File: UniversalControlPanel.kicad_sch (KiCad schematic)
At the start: 46 parts, among them J1 USB_B_Micro, J10 Conn_01x02, J11 Conn_01x02, J2 Conn_ARM_JTAG_SWD_10, J3 Conn_01x40, J4 Conn_02x03_Odd_Even, J5 Conn_01x02, J6 1Wire, J7 Conn_01x06, J8 Conn_01x07, J9 Conn_01x02, SW1 SW_Push, U1 TSR_1-2450, U2 MAX14783ExS, U3 USBLC6-2SC6, U4 AMS1117-3.3, U5 SN65HVD230, U6 ESP32-S2-WROOM-I

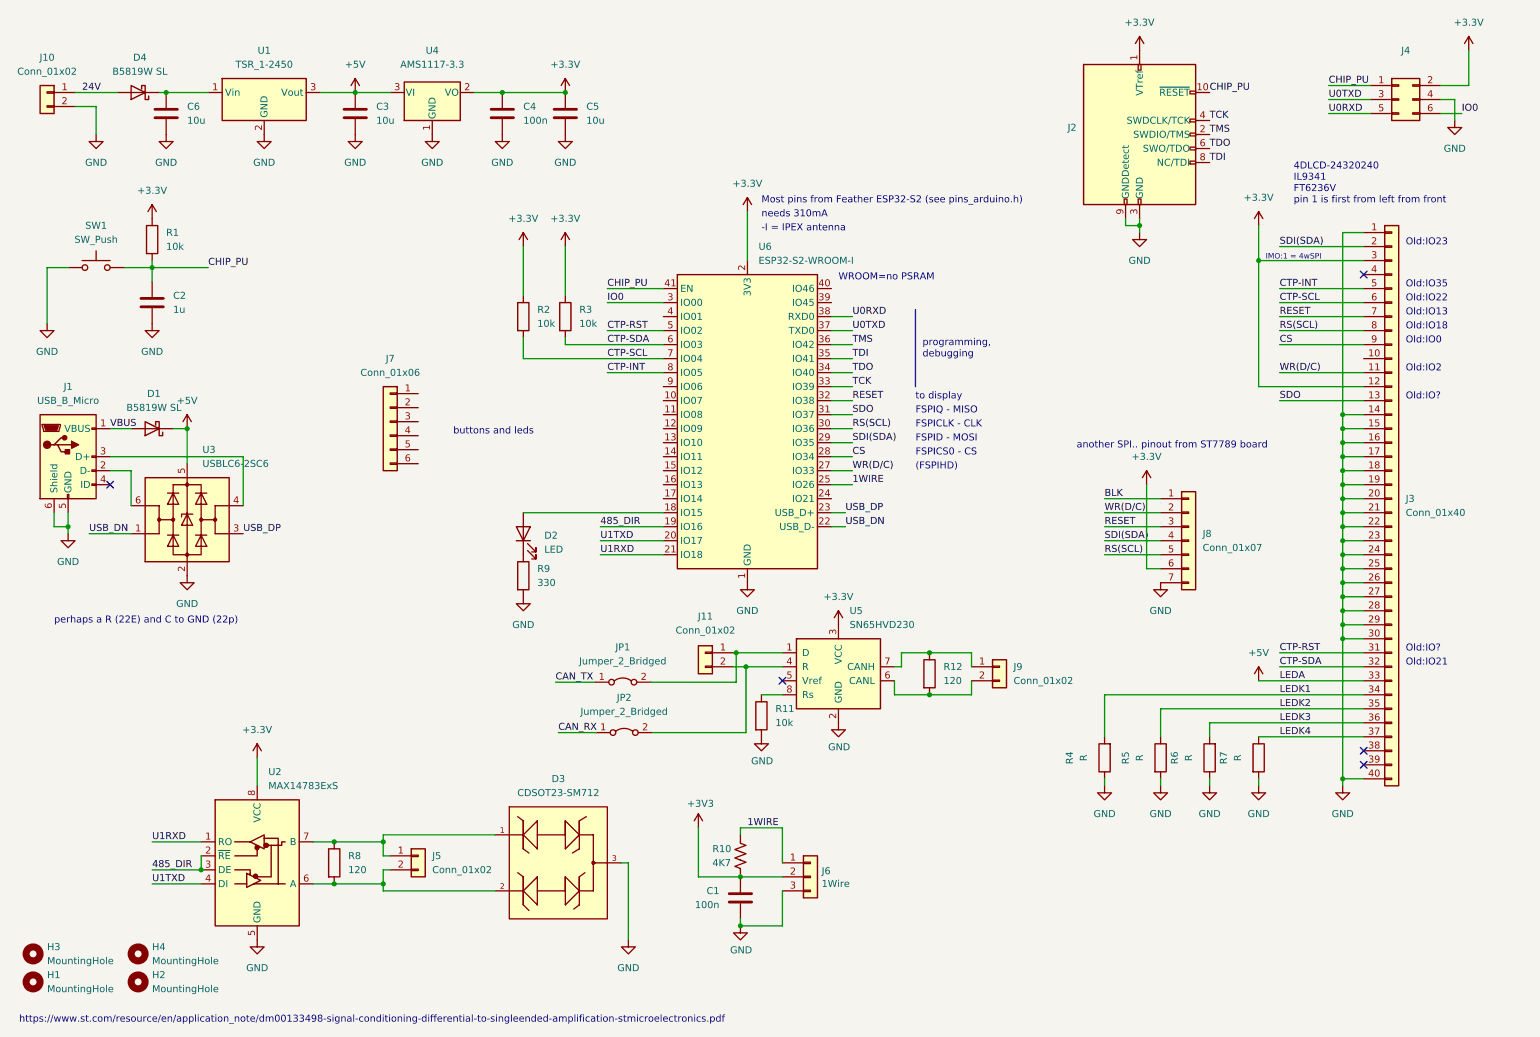
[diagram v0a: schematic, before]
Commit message: restart work
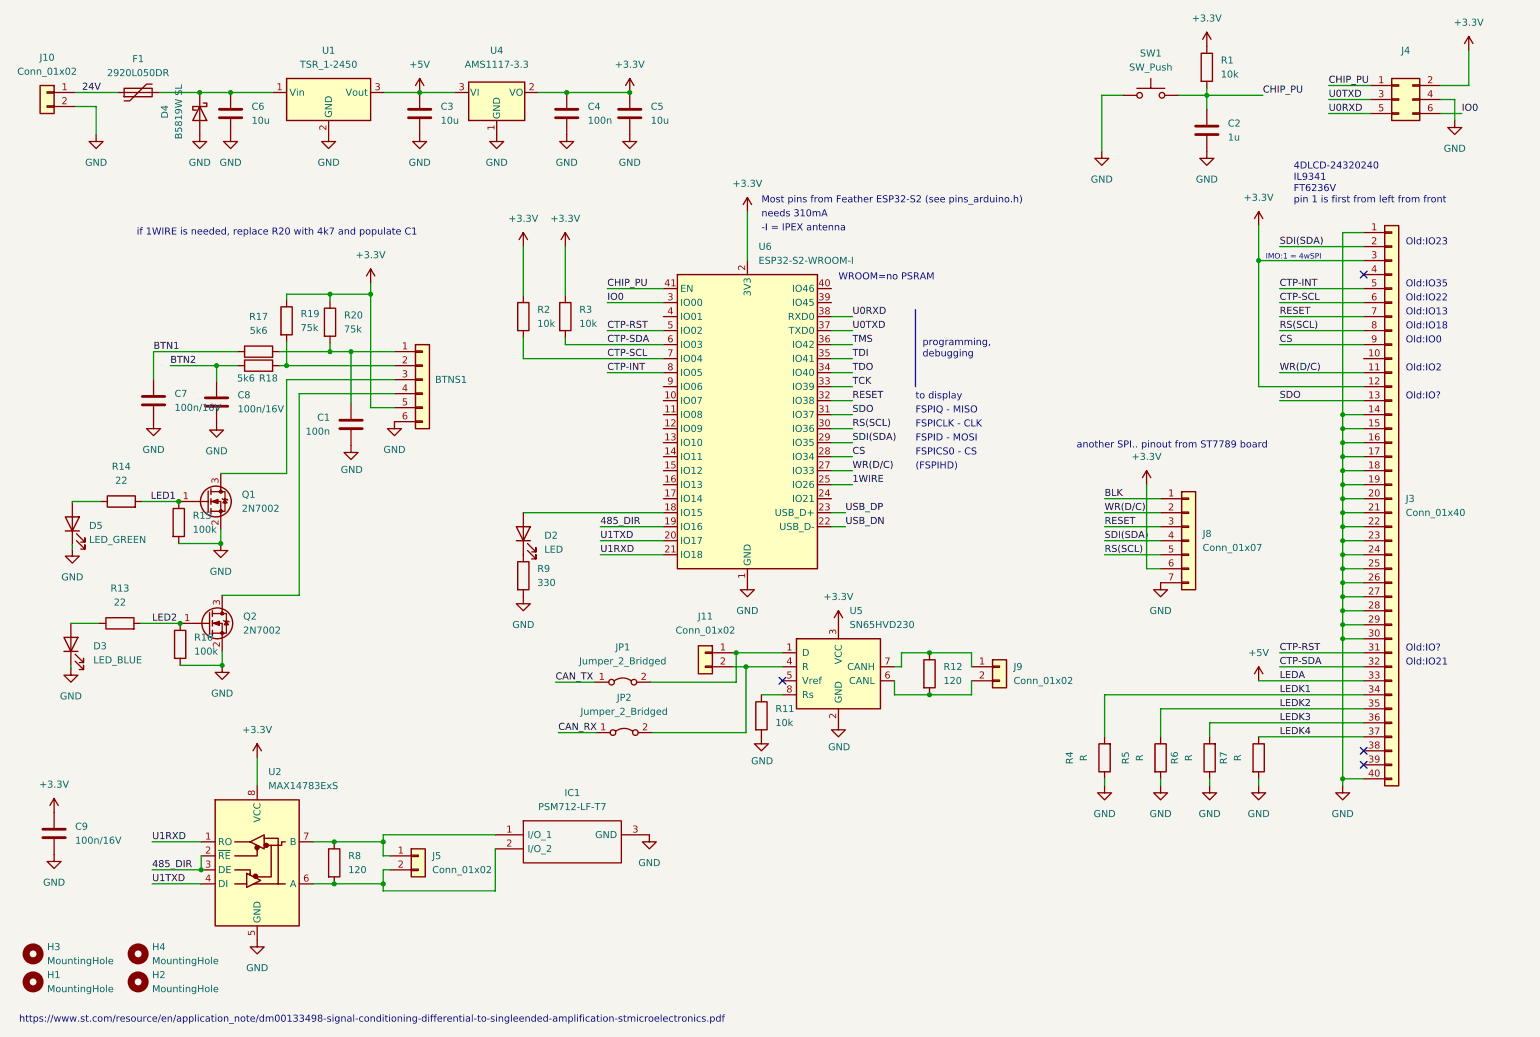
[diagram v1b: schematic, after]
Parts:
- removed D1: B5819W SL, Diode_SMD:D_SOD-123, symbol Device:D_Schottky
- removed D3: CDSOT23-SM712, Octopart:Bourns_Inc.-SOT23-0-0-IPC_B, symbol Octopart:CDSOT23-SM712
- removed J1: USB_B_Micro, Connector_USB:USB_Mini-B_Tensility_54-00023_Vertical, symbol Connector:USB_B_Micro
- removed J2: Conn_ARM_JTAG_SWD_10, Connector_PinHeader_1.27mm:PinHeader_2x05_P1.27mm_Vertical, symbol Connector:Conn_ARM_JTAG_SWD_10
- removed J6: 1Wire, Connector_PinHeader_2.54mm:PinHeader_1x03_P2.54mm_Vertical, symbol Connector_Generic:Conn_01x03
- removed J7: Conn_01x06, symbol Connector_Generic:Conn_01x06
- removed R10: 4K7, Resistor_SMD:R_0402_1005Metric, symbol Device:R_US
- removed U3: USBLC6-2SC6, Package_TO_SOT_SMD:SOT-23-6, symbol Power_Protection:USBLC6-2SC6
- added BTNS1: Conn_01x06, Connector_JST:JST_XH_B6B-XH-A_1x06_P2.50mm_Vertical, symbol Connector_Generic:Conn_01x06
- added C7, C8, C9: 100n/16V, Capacitor_SMD:C_0402_1005Metric, symbol Device:C
- added D3: LED_BLUE, LED_SMD:LED_0603_1608Metric, symbol Device:LED
- added D5: LED_GREEN, LED_SMD:LED_0603_1608Metric, symbol Device:LED
- added F1: 2920L050DR, Fuse:Fuse_2920_7451Metric, symbol Device:Polyfuse
- added IC1: PSM712-LF-T7, Package_TO_SOT_SMD:SOT-23, symbol _Local:PSM712-LF-T7
- added Q1, Q2: 2N7002, Package_TO_SOT_SMD:SOT-23, symbol Transistor_FET:2N7002
- added R13, R14: 22, Resistor_SMD:R_0402_1005Metric, symbol Device:R
- added R15, R16: 100k, Resistor_SMD:R_0402_1005Metric, symbol Device:R
- added R17, R18: 5k6, Resistor_SMD:R_0402_1005Metric, symbol Device:R
- added R19, R20: 75k, Resistor_SMD:R_0402_1005Metric, symbol Device:R
- C1: now left out of the parts list
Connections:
- net +3V3: now also BTNS1.5 (Pin_5), C9.1, R19.1, R20.1; no longer C1.2
- net 24V: now also F1.1; no longer D4.2 (A)
- net GND: now also D4.2 (A), BTNS1.6 (Pin_6), C7.2, C8.2, C9.2, D3.1 (K), D5.1 (K), IC1.3 (GND), Q1.2 (S), Q2.2 (S), R15.2, R16.2
- net at J5.1 (Pin_1), R8.1, U2.7 (B): now also IC1.1 (I/O_1)
- net at J5.2 (Pin_2), R8.2, U2.6 (A): now also IC1.2 (I/O_2)
- net at C6.1, D4.1 (K), U1.1 (Vin): now also F1.2
- new net: BTNS1.2 (Pin_2), R18.2, R19.2
- new net: BTNS1.1 (Pin_1), C1.2, R17.2, R20.2
- new net: D5.2 (A), R14.1
- new net: BTNS1.4 (Pin_4), Q2.3 (D)
- new net: BTNS1.3 (Pin_3), Q1.3 (D)
- new net: D3.2 (A), R13.1
- new net BTN1: C7.1, R17.1
- new net BTN2: C8.1, R18.1
- new net LED1: Q1.1 (G), R14.2, R15.1
- new net LED2: Q2.1 (G), R13.2, R16.1
- no-connect marks 5 -> 4
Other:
- note added: "if 1WIRE is needed, replace R20 with 4k7 and populate C1"
- note removed: "buttons and leds"
- note removed: "perhaps a R (22E) and C to GND (22p)"
- moved on the sheet: C2, C3, C4, C5, C6, D4, R1, SW1, U1, U4
